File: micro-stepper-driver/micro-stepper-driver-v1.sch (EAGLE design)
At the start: 3 parts

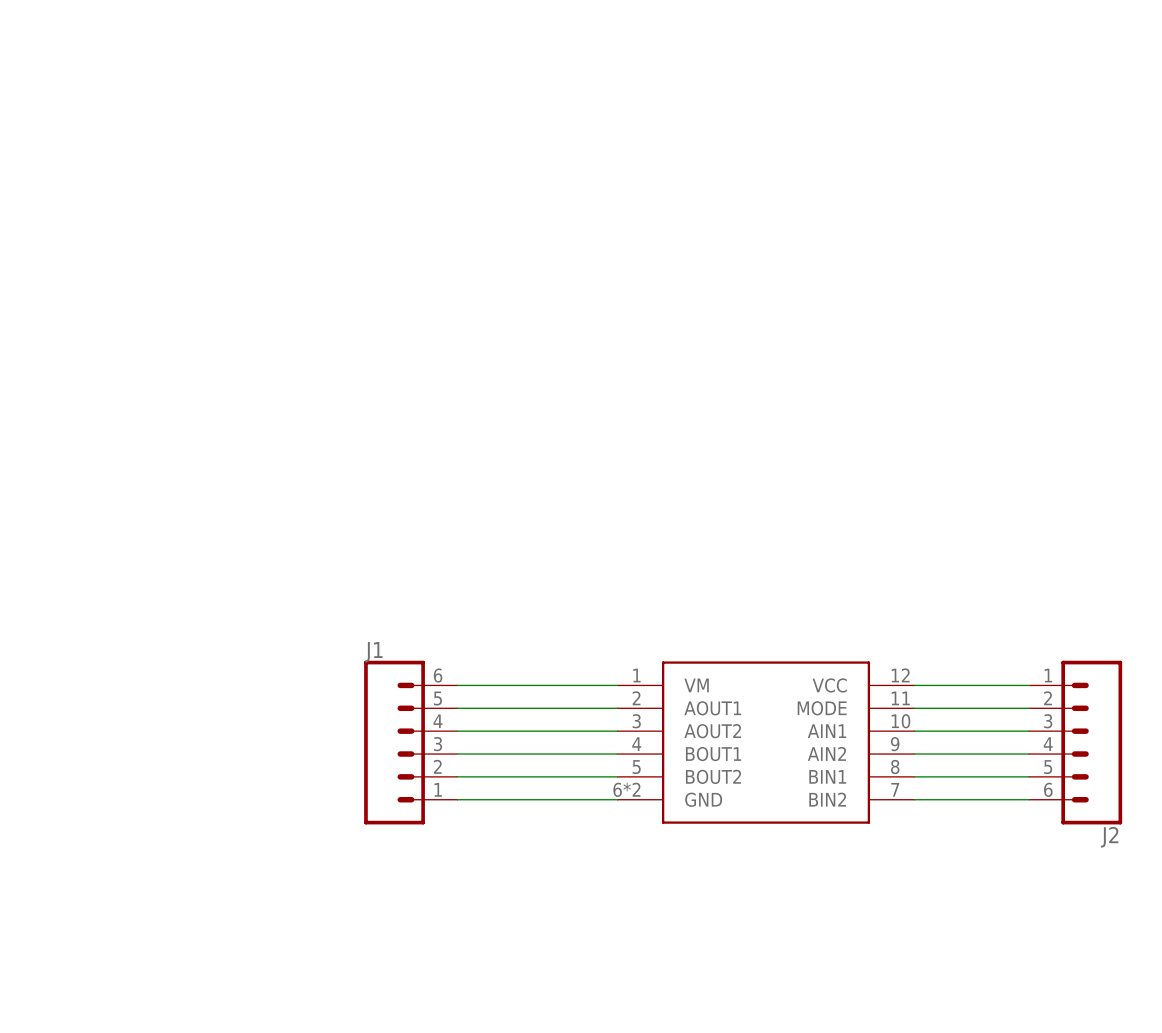
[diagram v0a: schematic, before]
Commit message: Micro driver
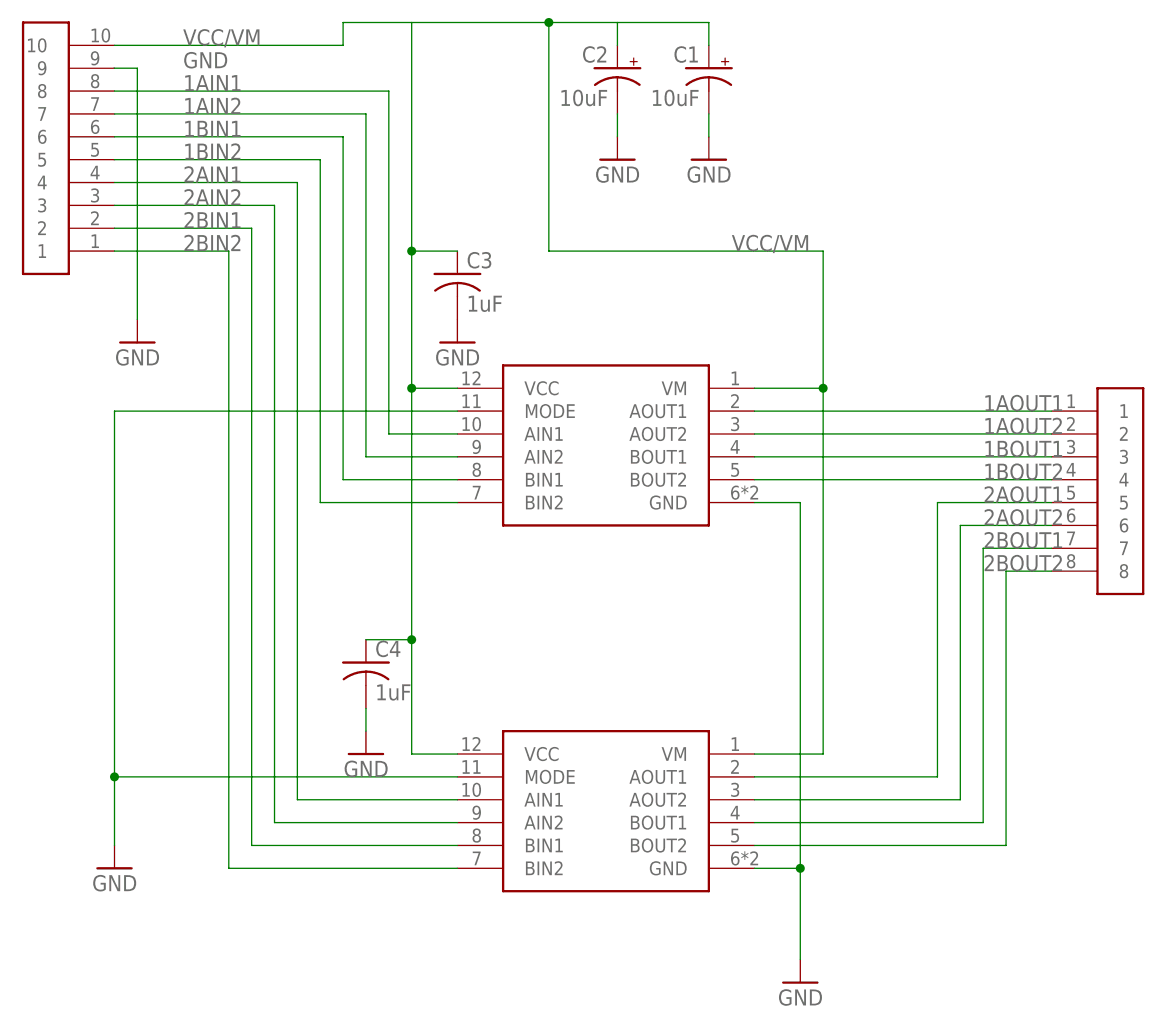
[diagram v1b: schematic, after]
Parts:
- removed J1, J2: (no value), SparkFun-Connectors:CONN_06SILK_FEMALE_PTH
- added C1, C2: 10uF, SparkFun-Capacitors:10UF-POLAR-EIA3216-16V-10%(TANT)
- added C3, C4: 1uF, resistor:C-USC0805K
- added U$2: EDGE_MOUNT_HEADER_X10, Ladvien_Eagle_Parts:EDGE_MOUNT_HEADER_X10
- added U$3: EDGE_MOUNT_HEAD_X8, Ladvien_Eagle_Parts:EDGE_MOUNT_HEAD_X8
- added U$4: DRV8835, Ladvien_Eagle_Parts:DRV8835
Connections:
- removed net N$1: J1.1, U$1.GND
- removed net N$10: J2.4, U$1.AIN2
- removed net N$11: J2.5, U$1.BIN1
- removed net N$12: J2.6, U$1.BIN2
- removed net N$2: J1.2, U$1.BOUT2
- removed net N$3: J1.3, U$1.BOUT1
- removed net N$4: J1.4, U$1.AOUT2
- removed net N$5: J1.5, U$1.AOUT1
- removed net N$6: J1.6, U$1.VM
- removed net N$7: J2.1, U$1.VCC
- removed net N$8: J2.2, U$1.MODE
- removed net N$9: J2.3, U$1.AIN1
- new net 1AIN1: U$2.8, U$4.AIN1
- new net 1AIN2: U$2.7, U$4.AIN2
- new net 1AOUT1: U$3.1, U$4.AOUT1
- new net 1AOUT2: U$3.2, U$4.AOUT2
- new net 1BIN1: U$2.6, U$4.BIN1
- new net 1BIN2: U$2.5, U$4.BIN2
- new net 1BOUT1: U$3.3, U$4.BOUT1
- new net 1BOUT2: U$3.4, U$4.BOUT2
- new net 2AIN1: U$1.AIN1, U$2.4
- new net 2AIN2: U$1.AIN2, U$2.3
- new net 2AOUT1: U$1.AOUT1, U$3.5
- new net 2AOUT2: U$1.AOUT2, U$3.6
- new net 2BIN1: U$1.BIN1, U$2.2
- new net 2BIN2: U$1.BIN2, U$2.1
- new net 2BOUT1: U$1.BOUT1, U$3.7
- new net 2BOUT2: U$1.BOUT2, U$3.8
- new net GND: C1.-, C2.-, C3.2, C4.2, U$1.GND, U$1.MODE, U$2.9, U$4.GND, U$4.MODE
- new net VCC/VM: C1.+, C2.+, C3.1, C4.1, U$1.VCC, U$1.VM, U$2.10, U$4.VCC, U$4.VM
